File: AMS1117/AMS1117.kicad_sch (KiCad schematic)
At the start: 0 parts

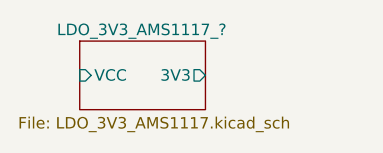
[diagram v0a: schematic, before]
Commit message: added gnd
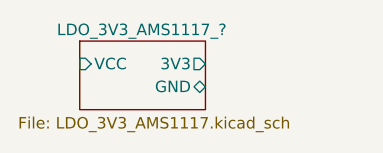
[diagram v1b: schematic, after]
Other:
- sheet LDO_3V3_AMS1117_? ports: added GND; removed none
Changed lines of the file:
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@@
 		)
 		(pin "3V3" output
-			(at 68.58 43.18 0)
+			(at 68.58 41.91 0)
 			(effects
 				(font
@@
 		)
 		(pin "VCC" input
-			(at 54.61 43.18 180)
+			(at 54.61 41.91 180)
 			(effects
 				(font
@@
 			)
 		)
+		(pin "GND" bidirectional
+			(at 68.58 44.45 0)
+			(effects
+				(font
+					(size 1.27 1.27)
+				)
+				(justify right)
+			)
+		)
